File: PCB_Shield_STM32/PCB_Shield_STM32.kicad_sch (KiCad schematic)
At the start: 8 parts, among them CN10 Conn_02x19_Odd_Even, CN11 Conn_01x02, CN12 Conn_01x02, CN5 Conn_01x10, CN6 Conn_01x08, CN7 Conn_02x19_Odd_Even, CN8 Conn_01x06, CN9 Conn_01x08

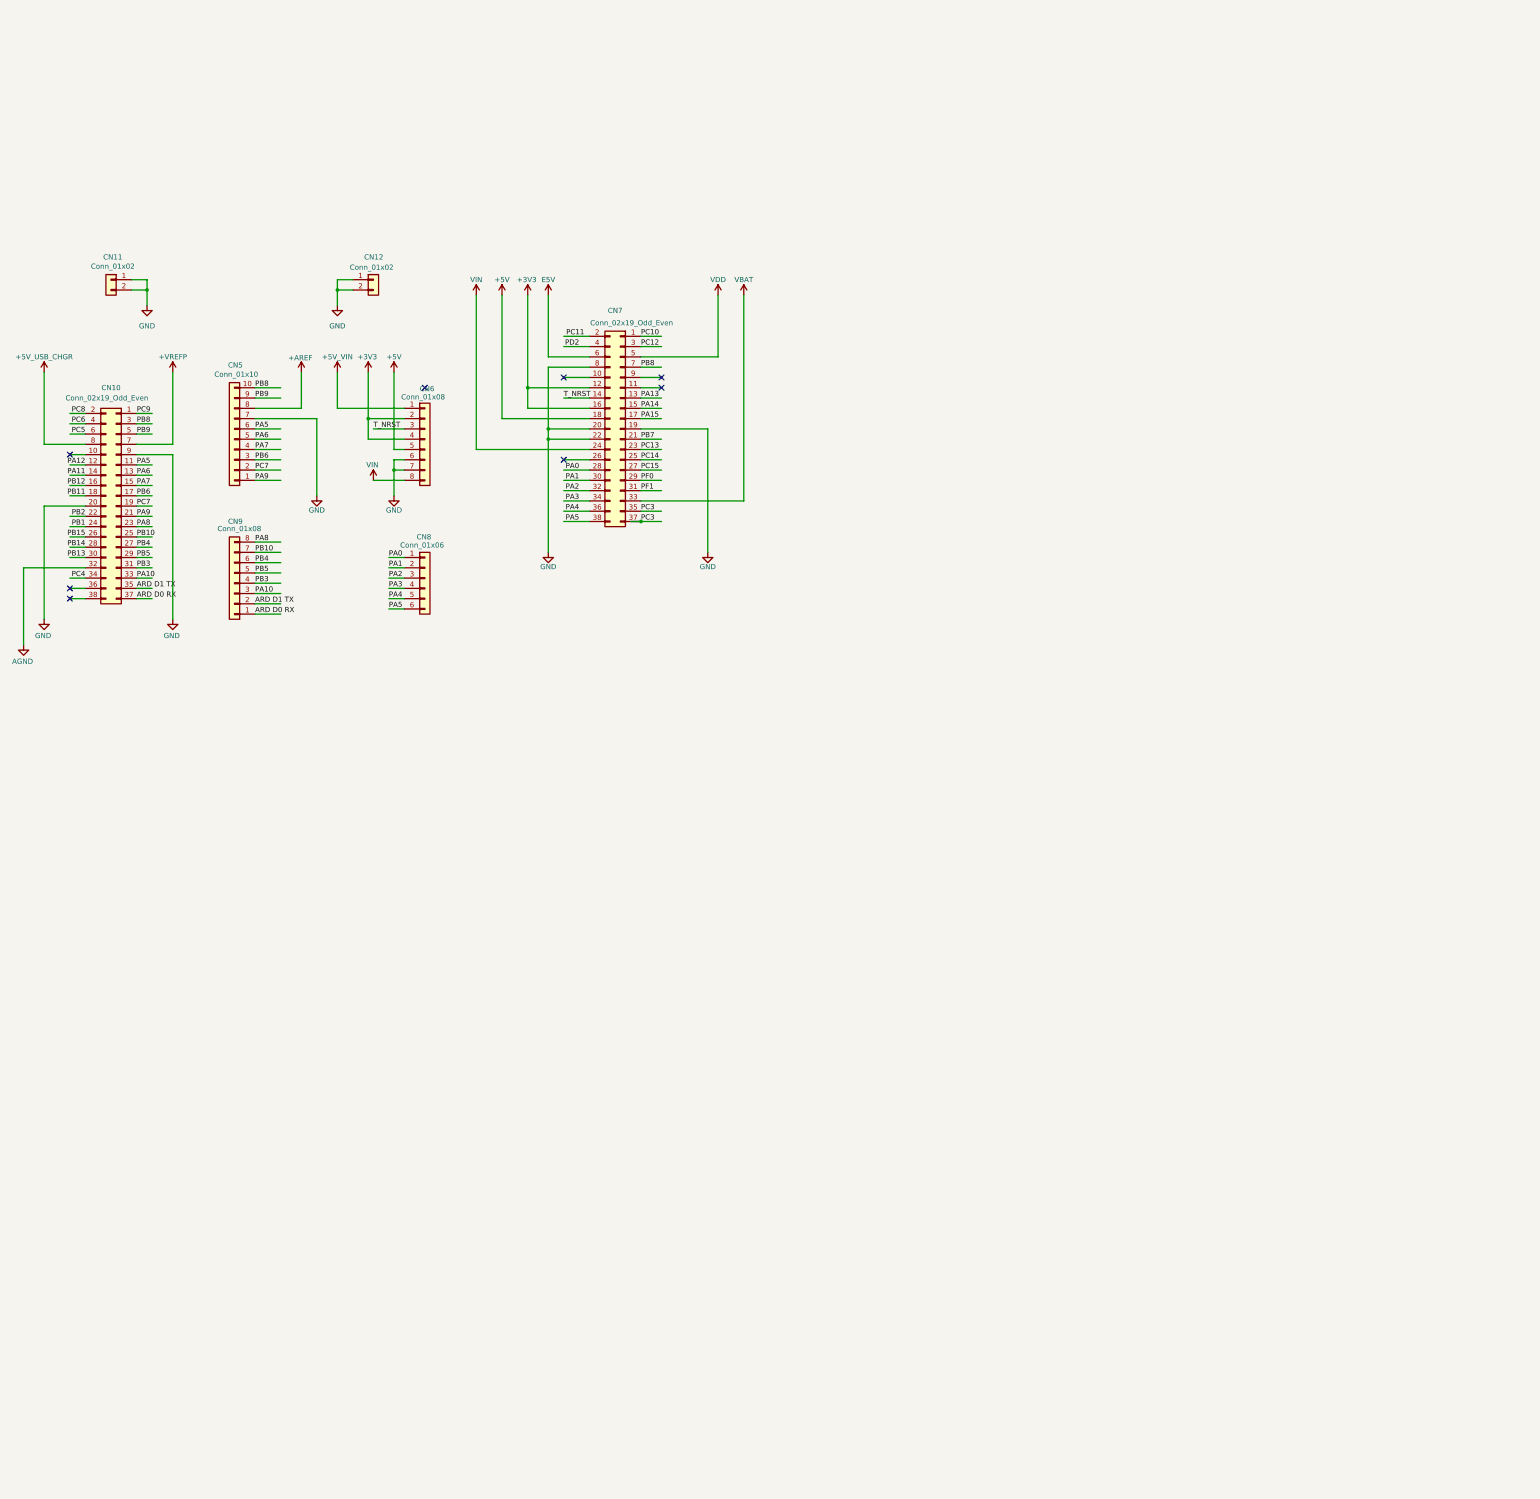
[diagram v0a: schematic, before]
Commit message: updated pcb.
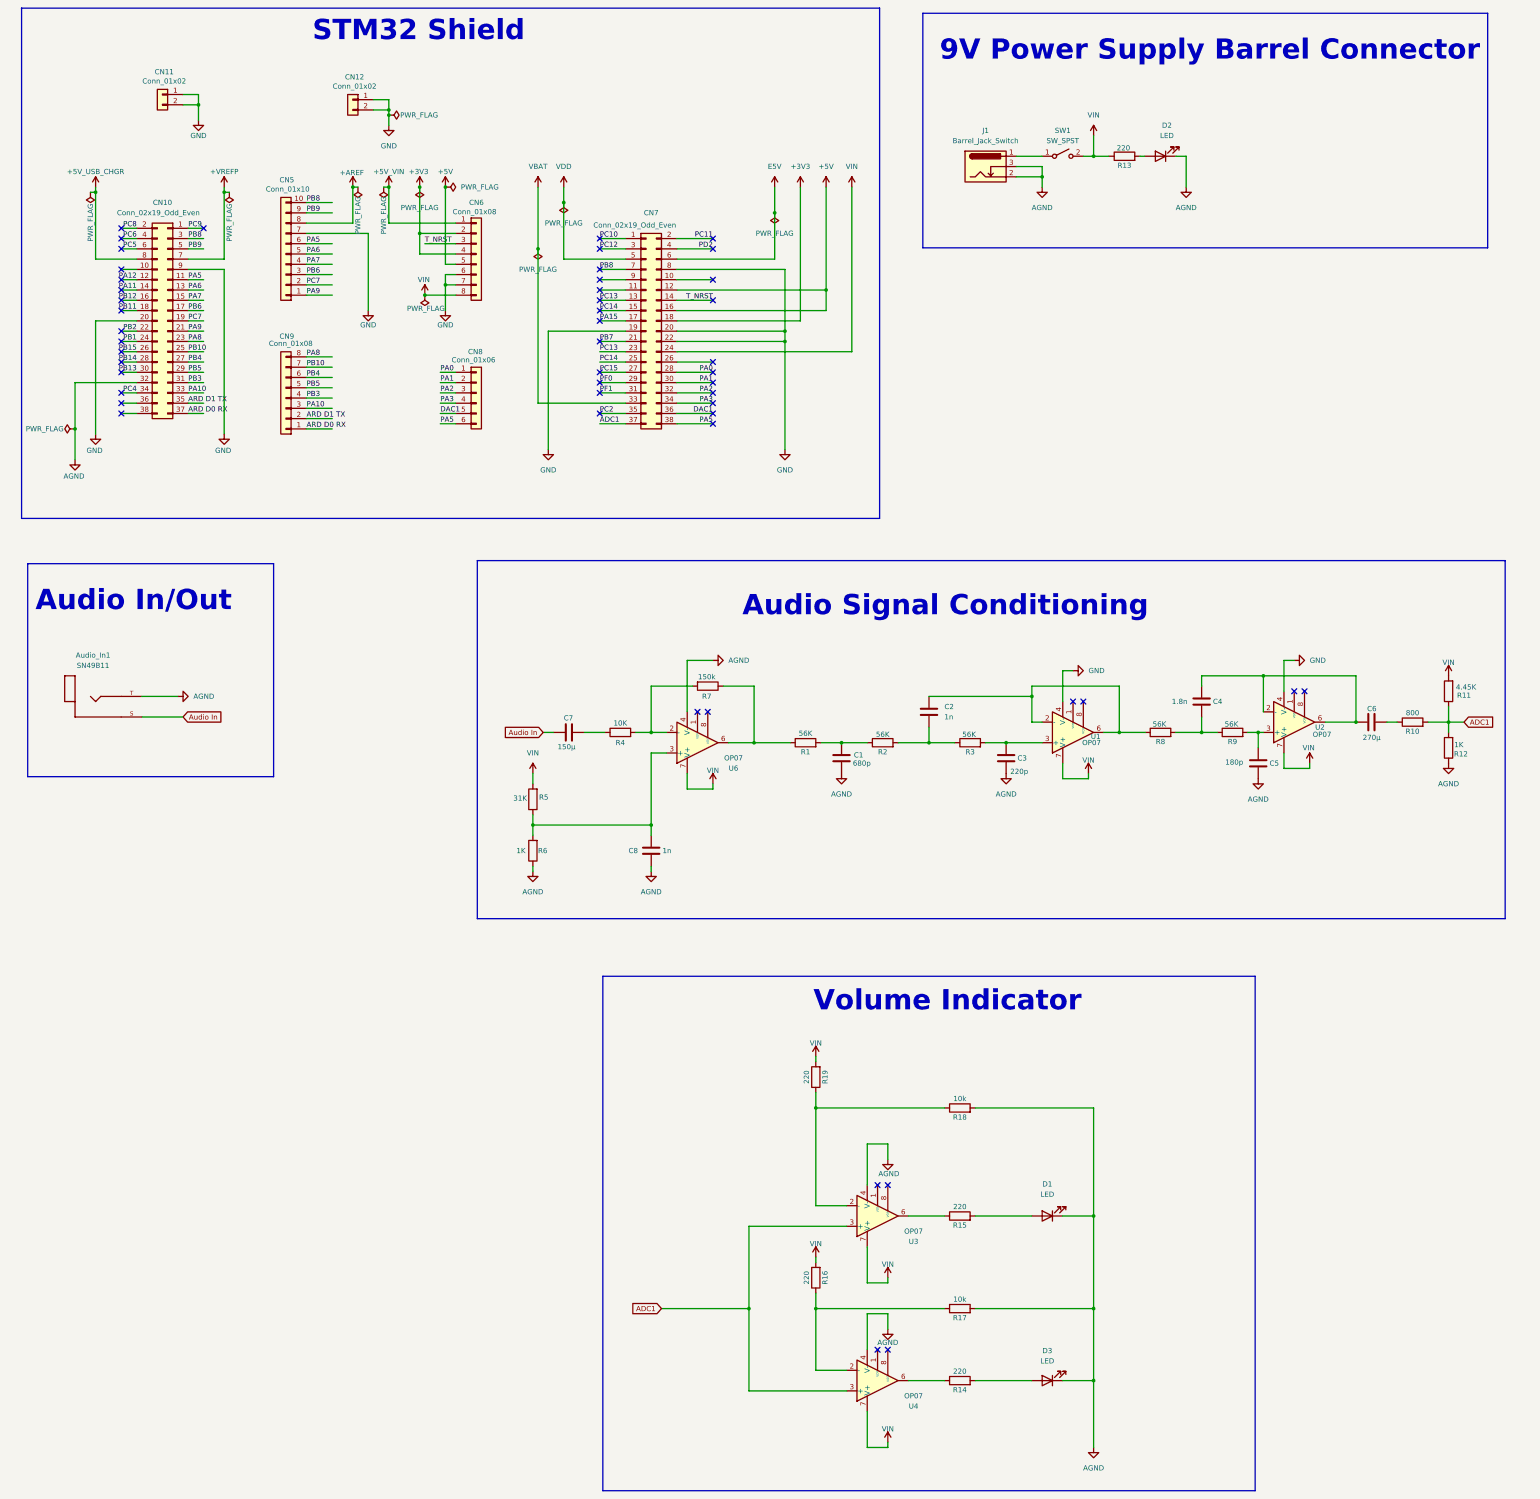
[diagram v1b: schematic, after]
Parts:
- added Audio_In1: SN49B11, SN49B11:SWITCHCRAFT_SN49B11, symbol SN49B11:SN49B11
- added C1: 680p, Capacitor_THT:C_Axial_L3.8mm_D2.6mm_P7.50mm_Horizontal, symbol Device:C
- added C2, C8: 1n, Capacitor_THT:C_Axial_L3.8mm_D2.6mm_P7.50mm_Horizontal, symbol Device:C
- added C3: 220p, Capacitor_THT:C_Axial_L3.8mm_D2.6mm_P7.50mm_Horizontal, symbol Device:C
- added C4: 1.8n, Capacitor_THT:C_Axial_L3.8mm_D2.6mm_P7.50mm_Horizontal, symbol Device:C
- added C5: 180p, Capacitor_THT:C_Axial_L3.8mm_D2.6mm_P7.50mm_Horizontal, symbol Device:C
- added C6: 270µ, Capacitor_THT:C_Axial_L3.8mm_D2.6mm_P7.50mm_Horizontal, symbol Device:C
- added C7: 150µ, Capacitor_THT:C_Axial_L3.8mm_D2.6mm_P7.50mm_Horizontal, symbol Device:C
- added D1, D2, D3: LED, LED_THT:LED_D3.0mm, symbol Device:LED
- added J1: Barrel_Jack_Switch, Connector_BarrelJack:BarrelJack_Horizontal, symbol Connector:Barrel_Jack_Switch
- added R1, R2, R3, R8, R9: 56K, Resistor_THT:R_Axial_DIN0204_L3.6mm_D1.6mm_P5.08mm_Horizontal, symbol Device:R
- added R10: 800, Resistor_THT:R_Axial_DIN0204_L3.6mm_D1.6mm_P5.08mm_Horizontal, symbol Device:R
- added R11: 4.45K, Resistor_THT:R_Axial_DIN0204_L3.6mm_D1.6mm_P5.08mm_Horizontal, symbol Device:R
- added R12, R6: 1K, Resistor_THT:R_Axial_DIN0204_L3.6mm_D1.6mm_P5.08mm_Horizontal, symbol Device:R
- added R13, R14, R15, R16, R19: 220, Resistor_THT:R_Axial_DIN0204_L3.6mm_D1.6mm_P5.08mm_Horizontal, symbol Device:R
- added R17, R18: 10k, Resistor_THT:R_Axial_DIN0204_L3.6mm_D1.6mm_P5.08mm_Horizontal, symbol Device:R
- added R4: 10K, Resistor_THT:R_Axial_DIN0204_L3.6mm_D1.6mm_P5.08mm_Horizontal, symbol Device:R
- added R5: 31K, Resistor_THT:R_Axial_DIN0204_L3.6mm_D1.6mm_P5.08mm_Horizontal, symbol Device:R
- added R7: 150k, Resistor_THT:R_Axial_DIN0204_L3.6mm_D1.6mm_P5.08mm_Horizontal, symbol Device:R
- added SW1: SW_SPST, Button_Switch_THT:SW_DIP_SPSTx01_Slide_9.78x4.72mm_W7.62mm_P2.54mm, symbol Switch:SW_SPST
- added U1, U2, U3, U4, U6: OP07, OP07DP:DIP794W45P254L959H508Q8, symbol Amplifier_Operational:OP07
- CN10, CN7: footprint (none) -> Connector_PinSocket_2.54mm:PinSocket_2x19_P2.54mm_Vertical
- CN11, CN12: footprint (none) -> Connector_PinSocket_2.54mm:PinSocket_1x02_P2.54mm_Vertical
- CN5: footprint (none) -> Connector_PinSocket_2.54mm:PinSocket_1x10_P2.54mm_Vertical
- CN6, CN9: footprint (none) -> Connector_PinSocket_2.54mm:PinSocket_1x08_P2.54mm_Vertical
- CN8: footprint (none) -> Connector_PinSocket_2.54mm:PinSocket_1x06_P2.54mm_Vertical
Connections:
- net PA13 is gone; now on net PC13: CN7.13 (Pin_13)
- net PA14 is gone; now on net PC14: CN7.15 (Pin_15)
- net +3V3: now also CN7.18 (Pin_18); no longer CN7.12 (Pin_12), CN7.16 (Pin_16)
- net +5V: now also CN7.12 (Pin_12), CN7.16 (Pin_16); no longer CN7.18 (Pin_18)
- net AGND: now also Audio_In1.T, C1.2, C3.2, C5.2, C8.2, D1.1 (K), D2.1 (K), D3.1 (K), J1.2, J1.3, R12.1, R17.2, R18.2, R6.1, U3.4 (V-), U4.4 (V-), U6.4 (V-)
- net GND: now also U1.4 (V-), U2.4 (V-)
- net VIN: now also R11.2, R13.1, R16.2, R19.2, R5.2, SW1.2 (B), U1.7 (V+), U2.7 (V+), U3.7 (V+), U4.7 (V+), U6.7 (V+)
- net PA4 renamed DAC1
- net PC3 renamed ADC1
- net ADC1: now also R10.2, R11.1, R12.2, U3.3 (+), U4.3 (+); no longer CN7.35 (Pin_35)
- new net: C7.1, R4.1
- new net: C8.1, R5.1, R6.2, U6.3 (+)
- new net: R15.1, U3.6
- new net: D1.2 (A), R15.2
- new net: R16.1, R17.1, U4.2 (-)
- new net: R14.1, U4.6
- new net: C4.2, R8.2, R9.1
- new net: C5.1, R9.2, U2.3 (+)
- new net: D2.2 (A), R13.2
- new net: C6.2, R10.1
- new net: C2.1, R8.1, U1.2 (-), U1.6
- new net: C2.2, R2.2, R3.1
- new net: D3.2 (A), R14.2
- new net: R4.2, R7.2, U6.2 (-)
- new net: R18.1, R19.1, U3.2 (-)
- new net: C3.1, R3.2, U1.3 (+)
- new net: C4.1, C6.1, U2.2 (-), U2.6
- new net: J1.1, SW1.1 (A)
- new net: R1.1, R7.1, U6.6
- new net: C1.1, R1.2, R2.1
- new net Audio In: Audio_In1.S, C7.2
- new net PC2: CN7.35 (Pin_35)
- no-connect marks 8 -> 51
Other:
- note added: "9V Power Supply Barrel Connector"
- note added: "Audio In/Out"
- note added: "Audio Signal Conditioning"
- note added: "STM32 Shield"
- note added: "Volume Indicator"
- company: (none) -> Noisey Boyz
- title: (none) -> ANC on STM32
- moved on the sheet: CN10, CN11, CN5, CN6, CN8, CN9
